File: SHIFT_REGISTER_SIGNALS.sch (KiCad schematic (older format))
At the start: 27 parts

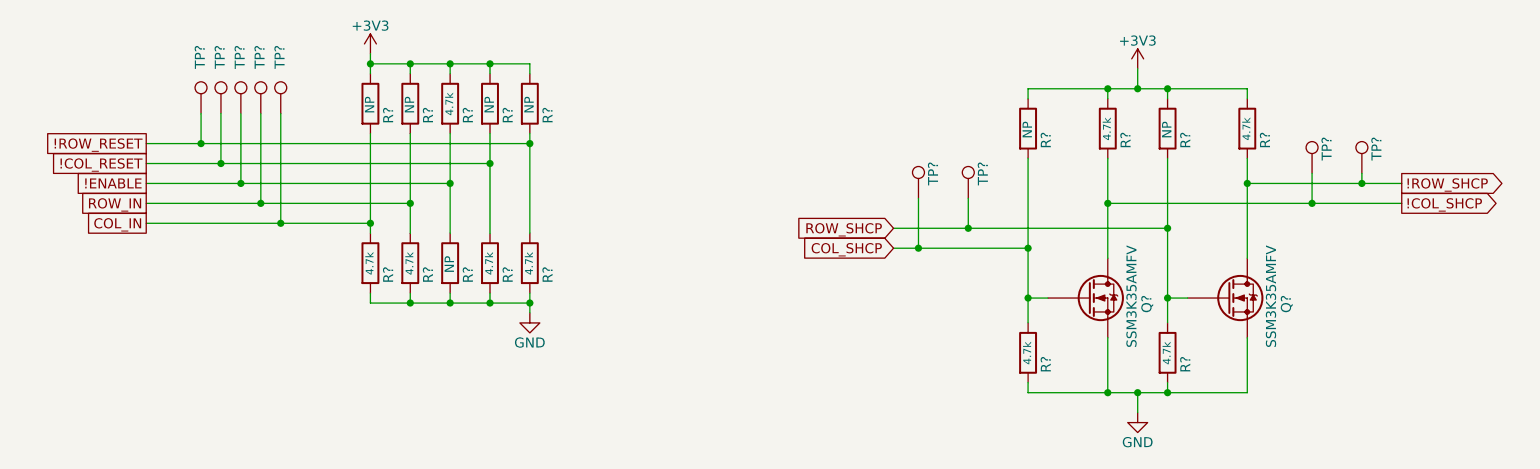
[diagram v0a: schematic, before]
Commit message: automated commit
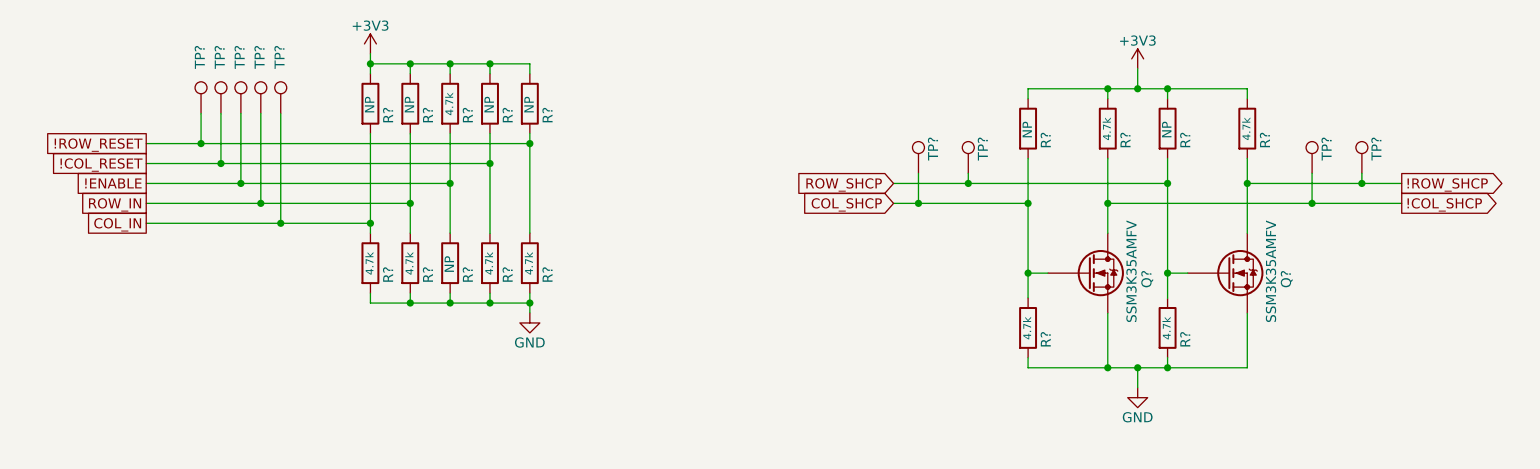
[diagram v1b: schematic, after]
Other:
- moved on the sheet: Q?, R?, TP?
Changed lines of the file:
@@
 L power:GND #PWR?
 U 1 1 5D4AE45E
-P 7775 4725
+P 7775 4600
 AR Path="/5D4AE45E" Ref="#PWR?"  Part="1"
 AR Path="/627E3ADC/5D4AE45E" Ref="#PWR?"  Part="1"
 AR Path="/620EB9A4/5D4AE45E" Ref="#PWR?"  Part="1"
 AR Path="/5D4A63FF/5D4AE45E" Ref="#PWR?"  Part="1"
-F 0 "#PWR?" H 7775 4475 50  0001 C CNN
-F 1 "GND" H 7775 4575 50  0000 C CNN
-F 2 "" H 7775 4725 50  0001 C CNN
-F 3 "" H 7775 4725 50  0001 C CNN
-	1    7775 4725
+F 0 "#PWR?" H 7775 4350 50  0001 C CNN
+F 1 "GND" H 7775 4450 50  0000 C CNN
+F 2 "" H 7775 4600 50  0001 C CNN
+F 3 "" H 7775 4600 50  0001 C CNN
+	1    7775 4600
 	1    0    0    -1
 $EndComp
@@
 Connection ~ 8325 3575
 Wire Wire Line
-	6550 3800 6925 3800
+	6550 3575 6925 3575
 Connection ~ 7625 3675
 Wire Wire Line
-	7625 4625 7625 4350
-Wire Wire Line
-	8325 4625 8325 4350
-Wire Wire Line
-	7225 4625 7625 4625
-Wire Wire Line
-	7925 4625 7925 4575
-Connection ~ 7925 4625
-Connection ~ 7625 4625
-Wire Wire Line
-	7225 4575 7225 4625
-Wire Wire Line
-	6550 3900 6675 3900
+	7625 4500 7625 4225
+Wire Wire Line
+	8325 4500 8325 4225
+Wire Wire Line
+	7225 4500 7625 4500
+Wire Wire Line
+	7925 4500 7925 4450
+Connection ~ 7925 4500
+Connection ~ 7625 4500
+Wire Wire Line
+	7225 4450 7225 4500
+Wire Wire Line
+	6550 3675 6675 3675
 Wire Wire Line
 	7225 3150 7225 3100
@@
 Connection ~ 7775 3100
 Wire Wire Line
-	7775 4625 7775 4725
-Connection ~ 7775 4625
-Wire Wire Line
-	6925 3650 6925 3800
-Connection ~ 6675 3900
-Wire Wire Line
-	6675 3650 6675 3900
-Connection ~ 6925 3800
+	7775 4500 7775 4600
+Connection ~ 7775 4500
+Wire Wire Line
+	6925 3525 6925 3575
+Connection ~ 6675 3675
+Wire Wire Line
+	6675 3525 6675 3675
+Connection ~ 6925 3575
 Connection ~ 8900 3575
 Wire Wire Line
@@
 	7925 3100 8325 3100
 Wire Wire Line
-	8325 3575 8325 3950
-Wire Wire Line
-	7625 3675 7625 3950
-Wire Wire Line
-	7925 4625 8325 4625
-Wire Wire Line
-	7625 4625 7775 4625
+	8325 3575 8325 3825
+Wire Wire Line
+	7625 3675 7625 3825
+Wire Wire Line
+	7925 4500 8325 4500
+Wire Wire Line
+	7625 4500 7775 4500
 Wire Wire Line
 	7775 3100 7925 3100
 Wire Wire Line
-	7775 4625 7925 4625
-Wire Wire Line
-	6675 3900 7225 3900
-Wire Wire Line
-	6925 3800 7925 3800
+	7775 4500 7925 4500
+Wire Wire Line
+	6675 3675 7225 3675
+Wire Wire Line
+	6925 3575 7925 3575
 Wire Wire Line
 	8900 3575 9100 3575
@@
 L custom:CRG0603F4K7 R?
 U 1 1 5D4AE511
-P 7925 4425
+P 7925 4300
 AR Path="/5D4AE511" Ref="R?"  Part="1"
 AR Path="/627E3ADC/5D4AE511" Ref="R?"  Part="1"
 AR Path="/620EB9A4/5D4AE511" Ref="R?"  Part="1"
 AR Path="/5D4A63FF/5D4AE511" Ref="R?"  Part="1"
-F 0 "R?" V 8045 4325 50  0000 L BNN
-F 1 "CRG0603F4K7" H 7175 3975 50  0001 L BNN
-F 2 "Resistor_SMD:R_0603_1608Metric" H 7175 3875 50  0001 L BNN
-F 3 "datasheets/PYu-RC_Group_51_RoHS_L_9.pdf" H 7175 3775 50  0001 L BNN
-F 4 "4.7k" V 7945 4365 39  0000 L BNN "Resistance"
-	1    7925 4425
+F 0 "R?" V 8045 4200 50  0000 L BNN
+F 1 "CRG0603F4K7" H 7175 3850 50  0001 L BNN
+F 2 "Resistor_SMD:R_0603_1608Metric" H 7175 3750 50  0001 L BNN
+F 3 "datasheets/PYu-RC_Group_51_RoHS_L_9.pdf" H 7175 3650 50  0001 L BNN
+F 4 "4.7k" V 7945 4240 39  0000 L BNN "Resistance"
+	1    7925 4300
 	1    0    0    -1
 $EndComp
@@
 L custom:CRG0603F4K7 R?
 U 1 1 5D4AE518
-P 7225 4425
+P 7225 4300
 AR Path="/5D4AE518" Ref="R?"  Part="1"
 AR Path="/627E3ADC/5D4AE518" Ref="R?"  Part="1"
 AR Path="/620EB9A4/5D4AE518" Ref="R?"  Part="1"
 AR Path="/5D4A63FF/5D4AE518" Ref="R?"  Part="1"
-F 0 "R?" V 7345 4325 50  0000 L BNN
-F 1 "CRG0603F4K7" H 6475 3975 50  0001 L BNN
-F 2 "Resistor_SMD:R_0603_1608Metric" H 6475 3875 50  0001 L BNN
-F 3 "datasheets/PYu-RC_Group_51_RoHS_L_9.pdf" H 6475 3775 50  0001 L BNN
-F 4 "4.7k" V 7245 4365 39  0000 L BNN "Resistance"
-	1    7225 4425
+F 0 "R?" V 7345 4200 50  0000 L BNN
+F 1 "CRG0603F4K7" H 6475 3850 50  0001 L BNN
+F 2 "Resistor_SMD:R_0603_1608Metric" H 6475 3750 50  0001 L BNN
+F 3 "datasheets/PYu-RC_Group_51_RoHS_L_9.pdf" H 6475 3650 50  0001 L BNN
+F 4 "4.7k" V 7245 4240 39  0000 L BNN "Resistance"
+	1    7225 4300
 	1    0    0    -1
 $EndComp
@@
 L custom:SSM3K35AMFV Q?
 U 1 1 5D4AE541
-P 7525 4150
+P 7525 4025
 AR Path="/5D4AE541" Ref="Q?"  Part="1"
 AR Path="/627E3ADC/5D4AE541" Ref="Q?"  Part="1"
 AR Path="/620EB9A4/5D4AE541" Ref="Q?"  Part="1"
 AR Path="/5D4A63FF/5D4AE541" Ref="Q?"  Part="1"
-F 0 "Q?" V 7850 4075 50  0000 L BNN
-F 1 "SSM3K35AMFV" V 7775 3900 50  0000 L BNN
-F 2 "" H 7725 4025 50  0001 L BIN
-F 3 "datasheets/SSM3K35AMFV.pdf" H 7725 4000 50  0001 L BNN
-	1    7525 4150
+F 0 "Q?" V 7850 3950 50  0000 L BNN
+F 1 "SSM3K35AMFV" V 7775 3775 50  0000 L BNN
+F 2 "" H 7725 3900 50  0001 L BIN
+F 3 "datasheets/SSM3K35AMFV.pdf" H 7725 3875 50  0001 L BNN
+	1    7525 4025
 	1    0    0    -1
 $EndComp
@@
 L custom:SSM3K35AMFV Q?
 U 1 1 5D4AE547
-P 8225 4150
+P 8225 4025
 AR Path="/5D4AE547" Ref="Q?"  Part="1"
 AR Path="/627E3ADC/5D4AE547" Ref="Q?"  Part="1"
 AR Path="/620EB9A4/5D4AE547" Ref="Q?"  Part="1"
 AR Path="/5D4A63FF/5D4AE547" Ref="Q?"  Part="1"
-F 0 "Q?" V 8550 4075 50  0000 L BNN
-F 1 "SSM3K35AMFV" V 8475 3900 50  0000 L BNN
-F 2 "" H 8425 4025 50  0001 L BIN
-F 3 "datasheets/SSM3K35AMFV.pdf" H 8425 4000 50  0001 L BNN
-	1    8225 4150
+F 0 "Q?" V 8550 3950 50  0000 L BNN
+F 1 "SSM3K35AMFV" V 8475 3775 50  0000 L BNN
+F 2 "" H 8425 3900 50  0001 L BIN
+F 3 "datasheets/SSM3K35AMFV.pdf" H 8425 3875 50  0001 L BNN
+	1    8225 4025
 	1    0    0    -1
 $EndComp
@@
 L Connector:TestPoint TP?
 U 1 1 5D4AE555
-P 6925 3650
+P 6925 3525
 AR Path="/5D4AE555" Ref="TP?"  Part="1"
 AR Path="/627E3ADC/5D4AE555" Ref="TP?"  Part="1"
 AR Path="/620EB9A4/5D4AE555" Ref="TP?"  Part="1"
 AR Path="/5D4A63FF/5D4AE555" Ref="TP?"  Part="1"
-F 0 "TP?" V 6850 3775 50  0000 C CNN
-F 1 "TestPoint" H 6675 3700 50  0001 C CNN
-F 2 "" H 7125 3650 50  0001 C CNN
-F 3 "~" H 7125 3650 50  0001 C CNN
-	1    6925 3650
+F 0 "TP?" V 6850 3650 50  0000 C CNN
+F 1 "TestPoint" H 6675 3575 50  0001 C CNN
+F 2 "" H 7125 3525 50  0001 C CNN
+F 3 "~" H 7125 3525 50  0001 C CNN
+	1    6925 3525
 	-1   0    0    -1
 $EndComp
@@
 L Connector:TestPoint TP?
 U 1 1 5D4AE55B
-P 6675 3650
+P 6675 3525
 AR Path="/5D4AE55B" Ref="TP?"  Part="1"
 AR Path="/627E3ADC/5D4AE55B" Ref="TP?"  Part="1"
 AR Path="/620EB9A4/5D4AE55B" Ref="TP?"  Part="1"
 AR Path="/5D4A63FF/5D4AE55B" Ref="TP?"  Part="1"
-F 0 "TP?" V 6600 3775 50  0000 C CNN
-F 1 "TestPoint" H 6425 3700 50  0001 C CNN
-F 2 "" H 6875 3650 50  0001 C CNN
-F 3 "~" H 6875 3650 50  0001 C CNN
-	1    6675 3650
+F 0 "TP?" V 6600 3650 50  0000 C CNN
+F 1 "TestPoint" H 6425 3575 50  0001 C CNN
+F 2 "" H 6875 3525 50  0001 C CNN
+F 3 "~" H 6875 3525 50  0001 C CNN
+	1    6675 3525
 	-1   0    0    -1
 $EndComp
@@
 Text GLabel 2800 3375 0    50   UnSpc ~ 0
 !ROW_RESET
-Text GLabel 6550 3800 0    50   Input ~ 0
+Text GLabel 6550 3575 0    50   Input ~ 0
 ROW_SHCP
-Text GLabel 6550 3900 0    50   Input ~ 0
+Text GLabel 6550 3675 0    50   Input ~ 0
 COL_SHCP
 Text GLabel 9100 3575 2    50   Output ~ 0
@@
 	8900 3525 8900 3575
 Wire Wire Line
-	7325 4150 7225 4150
-Connection ~ 7225 4150
-Wire Wire Line
-	7225 4150 7225 4275
-Wire Wire Line
-	8025 4150 7925 4150
-Connection ~ 7925 4150
-Wire Wire Line
-	7925 4150 7925 4275
-Connection ~ 7225 3900
-Wire Wire Line
-	7225 3900 7225 4150
-Connection ~ 7925 3800
-Wire Wire Line
-	7925 3800 7925 4150
-Wire Wire Line
-	7925 3450 7925 3800
-Wire Wire Line
-	7225 3450 7225 3900
+	7325 4025 7225 4025
+Connection ~ 7225 4025
+Wire Wire Line
+	7225 4025 7225 4150
+Wire Wire Line
+	8025 4025 7925 4025
+Connection ~ 7925 4025
+Wire Wire Line
+	7925 4025 7925 4150
+Wire Wire Line
+	7925 3450 7925 3575
+Wire Wire Line
+	7225 3450 7225 3675
+Connection ~ 7225 3675
+Connection ~ 7925 3575
+Wire Wire Line
+	7225 3675 7225 4025
+Wire Wire Line
+	7925 3575 7925 4025
 $EndSCHEMATC
